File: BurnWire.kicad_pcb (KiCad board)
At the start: 2 copper layers, 44.6 x 45.3 mm, 14 parts, among them J1 B6B-XH-A_LF__SN_, U1 ADP2303ARDZ

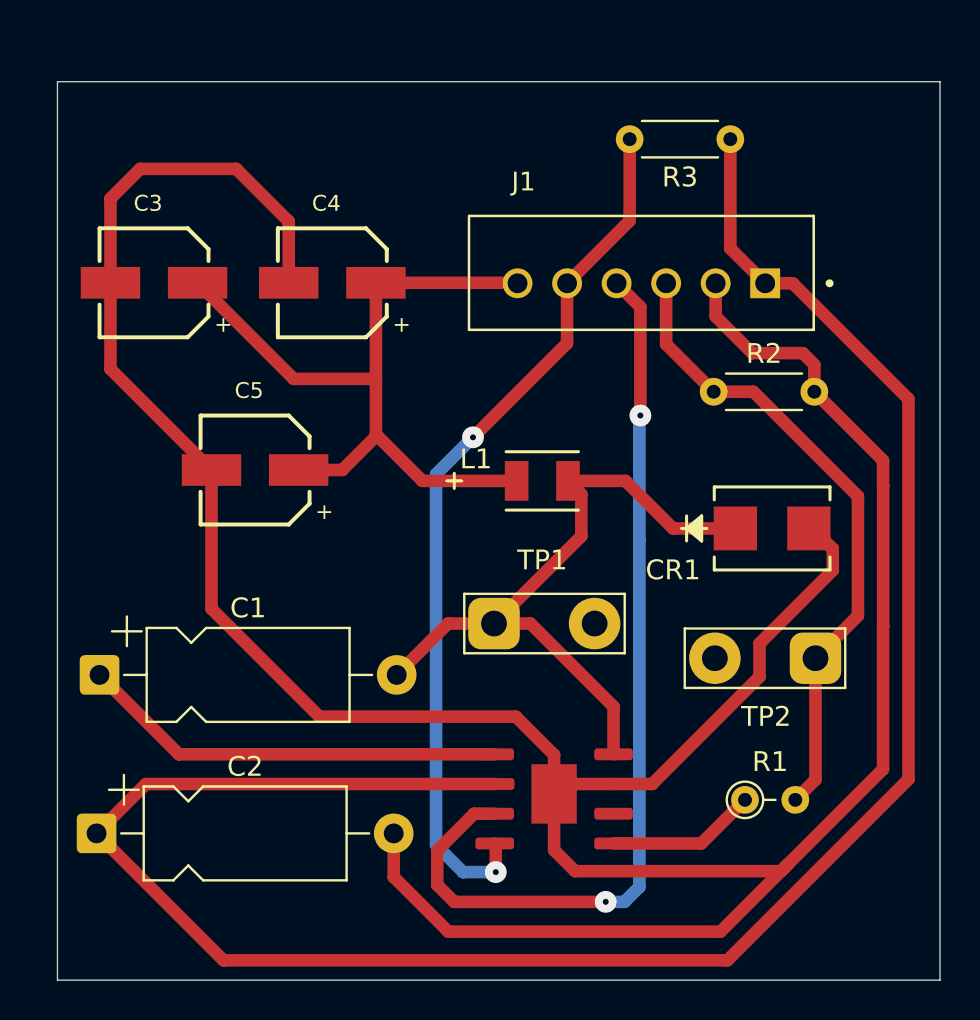
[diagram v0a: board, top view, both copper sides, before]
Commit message: done layout
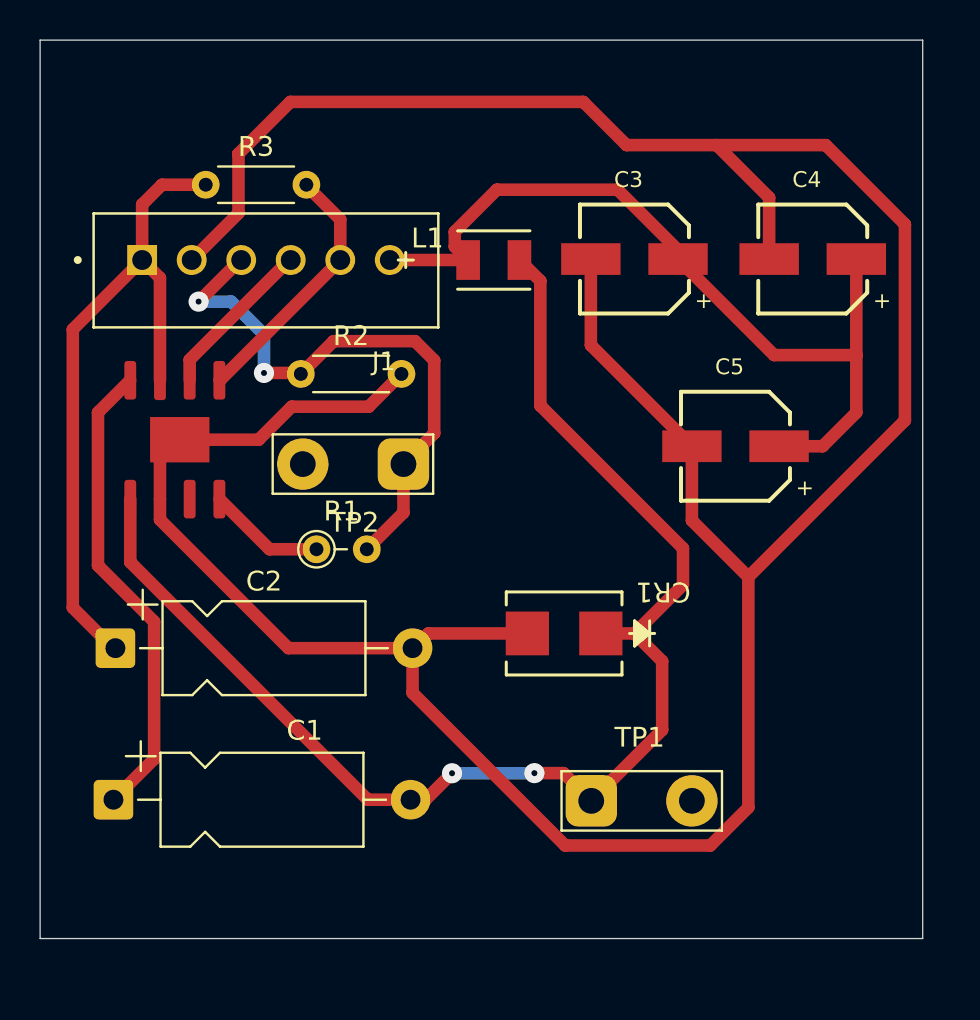
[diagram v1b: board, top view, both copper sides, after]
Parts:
- moved R3 26.6 mm to (139.1, 75.4), turned to 0 degrees
- moved U1 26.0 mm to (137.8, 88.3), turned to -90 degrees
- moved R1 25.1 mm to (144.7, 93.8)
- moved C3 24.3 mm to (160.8, 79.2)
- moved C4 24.3 mm to (169.8, 79.2)
- moved C5 24.3 mm to (165.8, 88.6)
- moved TP2 23.0 mm to (149.1, 89.5)
- moved R2 20.9 mm to (143.9, 85.0)
- moved J1 19.0 mm to (142.2, 79.7), turned to 180 degrees
- moved CR1 11.8 mm to (157.2, 98.0), turned to 180 degrees
- moved L1 11.4 mm to (153.7, 79.2)
- moved TP1 10.2 mm to (158.6, 106.5)
- moved C2 9.40 mm to (134.6, 98.8)
- moved C1 6.34 mm to (134.4, 106.4)
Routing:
- net /VBatt: track 105.4 -> 34.9 mm
- net /EN: track 47.2 -> 8.22 mm, vias 2 -> 0
- net Net-(U1-SW): track 34.9 -> 68.0 mm, vias 0 -> 2
- net Net-(U1-PGOOD): track 44.7 -> 13.1 mm, vias 2 -> 0
- net GND: track 159.1 -> 165.0 mm
- net /Vout: track 38.6 -> 42.9 mm
- net /VCutN: track 32.6 -> 29.6 mm, vias 0 -> 2
- net Net-(U1-BST): track 21.6 -> 23.9 mm
- net Net-(U1-FB): track 7.55 -> 5.95 mm
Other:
- board size 44.6 x 45.3 mm -> 44.6 x 45.4 mm
